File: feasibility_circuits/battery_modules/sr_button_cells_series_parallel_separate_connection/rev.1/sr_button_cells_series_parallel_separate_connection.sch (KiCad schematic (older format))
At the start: 25 parts, among them J1 Batt Out, J10 CONN_01X01, J11 CONN_01X01, J12 CONN_01X01, J13 CONN_01X01, J14 CONN_01X01, J15 Parallel, J16 Series, J17 Cell2, J18 Cell1, J19 CONN_01X01, J2 Batt Out, J20 Parallel, J21 CONN_01X01, J22 CONN_01X01, J23 CONN_01X01, J3 CONN_01X01, J4 CONN_01X01, J5 CONN_01X01, J6 CONN_01X01, J7 Jumper, J8 Jumper, J9 CONN_01X01

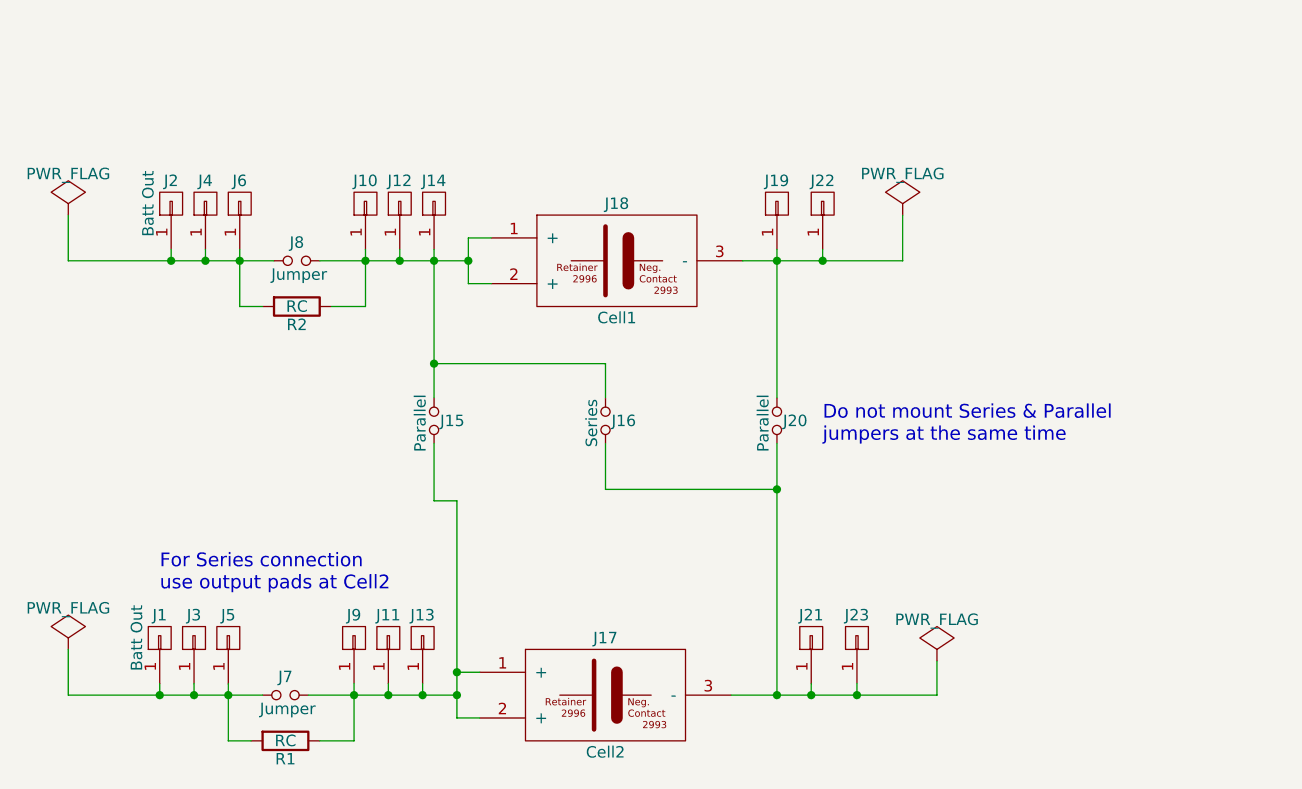
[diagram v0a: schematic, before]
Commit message: Added files forgotten in last commit.
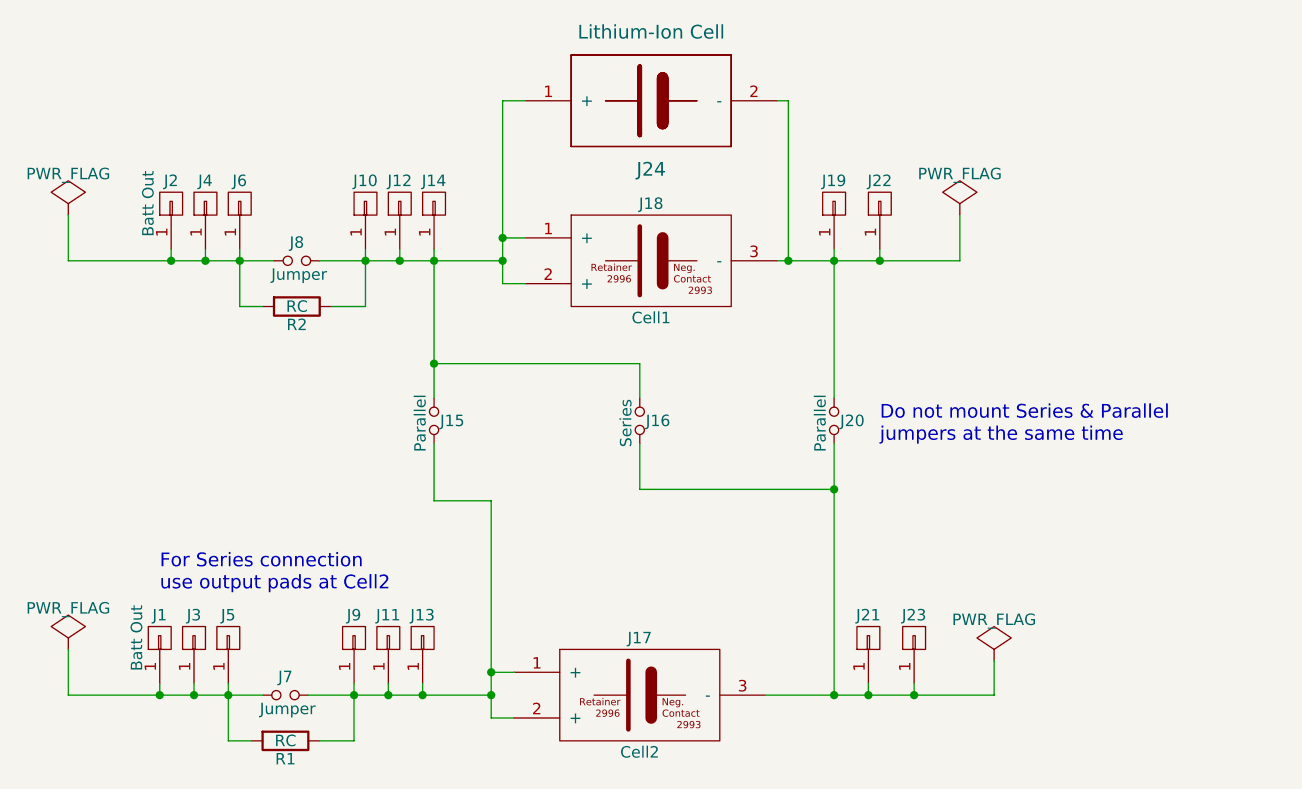
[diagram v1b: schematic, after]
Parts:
- added J24: Lithium-Ion Cell, Custom Battery Products:proto_button_cell_holder-smd-498, symbol BUTTON_CELL_HOLDER/SMD/11.6MM/498
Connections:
- net at J10.1 (P1), J12.1 (P1), J14.1 (P1)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: now also J24.1 (+)
- net at J18.3 (-), J19.1 (P1), J20.1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: now also J24.2 (-)
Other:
- moved on the sheet: J16, J17, J18, J19, J20, J21, J22, J23
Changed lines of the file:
@@
 L BUTTON_CELL_HOLDER/SMD/11.6MM/2996/2993 J18
 U 1 1 5902EBB9
-P 6300 2500
-F 0 "J18" H 6300 2750 50  0000 C CNN
-F 1 "Cell1" H 6300 2250 50  0000 C CNN
-F 2 "Custom Battery Products:proto_button_cell_holder-smd-2996-2993" H 6300 2500 60  0001 C CNN
-F 3 "" H 6300 2500 60  0001 C CNN
-	1    6300 2500
+P 6450 2500
+F 0 "J18" H 6450 2750 50  0000 C CNN
+F 1 "Cell1" H 6450 2250 50  0000 C CNN
+F 2 "Custom Battery Products:proto_button_cell_holder-smd-2996-2993" H 6450 2500 60  0001 C CNN
+F 3 "" H 6450 2500 60  0001 C CNN
+	1    6450 2500
 	1    0    0    -1
 $EndComp
@@
 L CONN_01X01 J19
 U 1 1 5902F107
-P 7000 2250
-F 0 "J19" V 7100 2250 50  0000 C CNN
-F 1 "CONN_01X01" V 7100 2250 50  0001 C CNN
-F 2 "Custom Connectors:proto_pad-square-3mm" H 7000 2250 50  0001 C CNN
-F 3 "" H 7000 2250 50  0000 C CNN
-	1    7000 2250
+P 7250 2250
+F 0 "J19" V 7350 2250 50  0000 C CNN
+F 1 "CONN_01X01" V 7350 2250 50  0001 C CNN
+F 2 "Custom Connectors:proto_pad-square-3mm" H 7250 2250 50  0001 C CNN
+F 3 "" H 7250 2250 50  0000 C CNN
+	1    7250 2250
 	0    -1   -1   0
 $EndComp
@@
 L CONN_01X01 J22
 U 1 1 5902F168
-P 7200 2250
-F 0 "J22" V 7300 2250 50  0000 C CNN
-F 1 "CONN_01X01" V 7300 2250 50  0001 C CNN
-F 2 "Custom Connectors:proto_pad-square-3mm" H 7200 2250 50  0001 C CNN
-F 3 "" H 7200 2250 50  0000 C CNN
-	1    7200 2250
+P 7450 2250
+F 0 "J22" V 7550 2250 50  0000 C CNN
+F 1 "CONN_01X01" V 7550 2250 50  0001 C CNN
+F 2 "Custom Connectors:proto_pad-square-3mm" H 7450 2250 50  0001 C CNN
+F 3 "" H 7450 2250 50  0000 C CNN
+	1    7450 2250
 	0    -1   -1   0
 $EndComp
@@
 L BUTTON_CELL_HOLDER/SMD/11.6MM/2996/2993 J17
 U 1 1 5902F4E4
-P 6250 4400
-F 0 "J17" H 6250 4650 50  0000 C CNN
-F 1 "Cell2" H 6250 4150 50  0000 C CNN
-F 2 "Custom Battery Products:proto_button_cell_holder-smd-2996-2993" H 6250 4400 60  0001 C CNN
-F 3 "" H 6250 4400 60  0001 C CNN
-	1    6250 4400
+P 6400 4400
+F 0 "J17" H 6400 4650 50  0000 C CNN
+F 1 "Cell2" H 6400 4150 50  0000 C CNN
+F 2 "Custom Battery Products:proto_button_cell_holder-smd-2996-2993" H 6400 4400 60  0001 C CNN
+F 3 "" H 6400 4400 60  0001 C CNN
+	1    6400 4400
 	1    0    0    -1
 $EndComp
@@
 L CONN_01X01 J21
 U 1 1 5902F508
-P 7150 4150
-F 0 "J21" V 7250 4150 50  0000 C CNN
-F 1 "CONN_01X01" V 7250 4150 50  0001 C CNN
-F 2 "Custom Connectors:proto_pad-square-3mm" H 7150 4150 50  0001 C CNN
-F 3 "" H 7150 4150 50  0000 C CNN
-	1    7150 4150
+P 7400 4150
+F 0 "J21" V 7500 4150 50  0000 C CNN
+F 1 "CONN_01X01" V 7500 4150 50  0001 C CNN
+F 2 "Custom Connectors:proto_pad-square-3mm" H 7400 4150 50  0001 C CNN
+F 3 "" H 7400 4150 50  0000 C CNN
+	1    7400 4150
 	0    -1   -1   0
 $EndComp
@@
 L CONN_01X01 J23
 U 1 1 5902F50E
-P 7350 4150
-F 0 "J23" V 7450 4150 50  0000 C CNN
-F 1 "CONN_01X01" V 7450 4150 50  0001 C CNN
-F 2 "Custom Connectors:proto_pad-square-3mm" H 7350 4150 50  0001 C CNN
-F 3 "" H 7350 4150 50  0000 C CNN
-	1    7350 4150
+P 7600 4150
+F 0 "J23" V 7700 4150 50  0000 C CNN
+F 1 "CONN_01X01" V 7700 4150 50  0001 C CNN
+F 2 "Custom Connectors:proto_pad-square-3mm" H 7600 4150 50  0001 C CNN
+F 3 "" H 7600 4150 50  0000 C CNN
+	1    7600 4150
 	0    -1   -1   0
 $EndComp
@@
 L Jumper_NO_Small J20
 U 1 1 5902FD72
-P 7000 3200
-F 0 "J20" V 7000 3280 50  0000 C CNN
-F 1 "Parallel" H 7010 3140 50  0000 C CNN
-F 2 "Custom Connectors:proto_header-vt-1x2-2.54mm-G_C__SABN_M30" H 7000 3200 50  0001 C CNN
-F 3 "" H 7000 3200 50  0000 C CNN
-	1    7000 3200
+P 7250 3200
+F 0 "J20" V 7250 3280 50  0000 C CNN
+F 1 "Parallel" H 7260 3140 50  0000 C CNN
+F 2 "Custom Connectors:proto_header-vt-1x2-2.54mm-G_C__SABN_M30" H 7250 3200 50  0001 C CNN
+F 3 "" H 7250 3200 50  0000 C CNN
+	1    7250 3200
 	0    1    1    0
 $EndComp
@@
 L Jumper_NO_Small J16
 U 1 1 5902FDEA
-P 6250 3200
-F 0 "J16" V 6250 3280 50  0000 C CNN
-F 1 "Series" H 6260 3140 50  0000 C CNN
-F 2 "Custom Connectors:proto_header-vt-1x2-2.54mm-G_C__SABN_M30" H 6250 3200 50  0001 C CNN
-F 3 "" H 6250 3200 50  0000 C CNN
-	1    6250 3200
+P 6400 3200
+F 0 "J16" V 6400 3280 50  0000 C CNN
+F 1 "Series" H 6410 3140 50  0000 C CNN
+F 2 "Custom Connectors:proto_header-vt-1x2-2.54mm-G_C__SABN_M30" H 6400 3200 50  0001 C CNN
+F 3 "" H 6400 3200 50  0000 C CNN
+	1    6400 3200
 	0    1    1    0
 $EndComp
-Text Notes 7200 3300 0    60   ~ 0
+Text Notes 7450 3300 0    60   ~ 0
 Do not mount Series & Parallel\njumpers at the same time
 Text Notes 4300 3950 0    60   ~ 0
 For Series connection\nuse output pads at Cell2
 Wire Wire Line
-	5750 2400 5650 2400
-Wire Wire Line
-	5650 2400 5650 2600
-Wire Wire Line
-	5650 2600 5750 2600
-Connection ~ 5650 2500
+	5900 2400 5800 2400
+Wire Wire Line
+	5800 1800 5800 2600
+Wire Wire Line
+	5800 2600 5900 2600
+Connection ~ 5800 2500
 Connection ~ 5500 2500
 Wire Wire Line
@@
 	4650 2700 4750 2700
 Wire Wire Line
-	6850 2500 7550 2500
-Wire Wire Line
-	7000 2450 7000 3100
-Wire Wire Line
-	7200 2500 7200 2450
-Connection ~ 7000 2500
-Wire Wire Line
-	5700 4300 5600 4300
-Wire Wire Line
-	5600 4500 5700 4500
-Connection ~ 5600 4400
+	7250 2450 7250 3100
+Wire Wire Line
+	7450 2500 7450 2450
+Connection ~ 7250 2500
+Wire Wire Line
+	5850 4300 5750 4300
+Wire Wire Line
+	5750 4500 5850 4500
+Connection ~ 5750 4400
 Wire Wire Line
 	3900 4400 4750 4400
@@
 Wire Wire Line
 	4600 4600 4700 4600
-Connection ~ 5600 4300
-Wire Wire Line
-	5600 3550 5600 4500
+Connection ~ 5750 4300
+Wire Wire Line
+	5750 3550 5750 4500
 Wire Wire Line
 	5500 3300 5500 3550
 Wire Wire Line
-	5500 3550 5600 3550
+	5500 3550 5750 3550
 Wire Wire Line
 	5500 2450 5500 3100
 Wire Wire Line
-	7150 4350 7150 4400
-Wire Wire Line
-	6800 4400 7700 4400
-Wire Wire Line
-	7350 4400 7350 4350
-Connection ~ 7150 4400
-Wire Wire Line
-	7000 3300 7000 4400
-Connection ~ 7000 4400
-Wire Wire Line
-	6250 3100 6250 2950
-Wire Wire Line
-	6250 2950 5500 2950
+	7400 4350 7400 4400
+Wire Wire Line
+	7600 4400 7600 4350
+Connection ~ 7400 4400
+Wire Wire Line
+	7250 3300 7250 4400
+Connection ~ 7250 4400
+Wire Wire Line
+	6400 2950 6400 3100
+Wire Wire Line
+	5500 2950 6400 2950
 Connection ~ 5500 2950
 Wire Wire Line
-	6250 3300 6250 3500
-Wire Wire Line
-	6250 3500 7000 3500
-Connection ~ 7000 3500
+	6400 3300 6400 3500
+Connection ~ 7250 3500
 $Comp
 L CONN_01X01 J2
@@
 L PWR_FLAG #FLG02
 U 1 1 5903141A
-P 7550 2300
-F 0 "#FLG02" H 7550 2395 50  0001 C CNN
-F 1 "PWR_FLAG" H 7550 2480 50  0000 C CNN
-F 2 "" H 7550 2300 50  0000 C CNN
-F 3 "" H 7550 2300 50  0000 C CNN
-	1    7550 2300
-	1    0    0    -1
-$EndComp
-Wire Wire Line
-	7550 2500 7550 2300
-Connection ~ 7200 2500
+P 7800 2300
+F 0 "#FLG02" H 7800 2395 50  0001 C CNN
+F 1 "PWR_FLAG" H 7800 2480 50  0000 C CNN
+F 2 "" H 7800 2300 50  0000 C CNN
+F 3 "" H 7800 2300 50  0000 C CNN
+	1    7800 2300
+	1    0    0    -1
+$EndComp
+Wire Wire Line
+	7800 2500 7800 2300
+Connection ~ 7450 2500
 Wire Wire Line
 	3900 2300 3900 2500
@@
 L PWR_FLAG #FLG04
 U 1 1 590315C4
-P 7700 4250
-F 0 "#FLG04" H 7700 4345 50  0001 C CNN
-F 1 "PWR_FLAG" H 7700 4430 50  0000 C CNN
-F 2 "" H 7700 4250 50  0000 C CNN
-F 3 "" H 7700 4250 50  0000 C CNN
-	1    7700 4250
-	1    0    0    -1
-$EndComp
-Wire Wire Line
-	7700 4400 7700 4250
-Connection ~ 7350 4400
+P 7950 4250
+F 0 "#FLG04" H 7950 4345 50  0001 C CNN
+F 1 "PWR_FLAG" H 7950 4430 50  0000 C CNN
+F 2 "" H 7950 4250 50  0000 C CNN
+F 3 "" H 7950 4250 50  0000 C CNN
+	1    7950 4250
+	1    0    0    -1
+$EndComp
+Wire Wire Line
+	7950 4400 7950 4250
+Connection ~ 7600 4400
 $Comp
 L CONN_01X01 J10
@@
 	5200 2700 5200 2450
 Wire Wire Line
-	5000 2500 5650 2500
+	5000 2500 5800 2500
 Wire Wire Line
 	5050 2700 5200 2700
@@
 	5450 4350 5450 4400
 Wire Wire Line
-	4950 4400 5600 4400
+	4950 4400 5750 4400
 Wire Wire Line
 	5300 4350 5300 4400
@@
 Wire Wire Line
 	5150 4600 5000 4600
+$Comp
+L BUTTON_CELL_HOLDER/SMD/11.6MM/498 J24
+U 1 1 59045D1C
+P 6450 1800
+F 0 "J24" H 6450 1500 60  0000 C CNN
+F 1 "Lithium-Ion Cell" H 6450 2100 60  0000 C CNN
+F 2 "Custom Battery Products:proto_button_cell_holder-smd-498" H 6450 1800 60  0001 C CNN
+F 3 "" H 6450 1800 60  0001 C CNN
+	1    6450 1800
+	1    0    0    -1
+$EndComp
+Wire Wire Line
+	7000 2500 7800 2500
+Wire Wire Line
+	6400 3500 7250 3500
+Wire Wire Line
+	6950 4400 7950 4400
+Wire Wire Line
+	5800 1800 5900 1800
+Connection ~ 5800 2400
+Wire Wire Line
+	7000 1800 7050 1800
+Wire Wire Line
+	7050 1800 7050 2500
+Connection ~ 7050 2500
 $EndSCHEMATC
